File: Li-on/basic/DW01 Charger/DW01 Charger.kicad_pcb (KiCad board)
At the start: 2 copper layers, 34.5 x 20.5 mm, 10 parts, among them J1 Pos Batt, J2 NEG Batt, J3 POS IN/OUT, J4 NEG IN/OUT, Q1 RE1C002UNTCL, Q2 RE1C001ZPTL, U1 DW01A

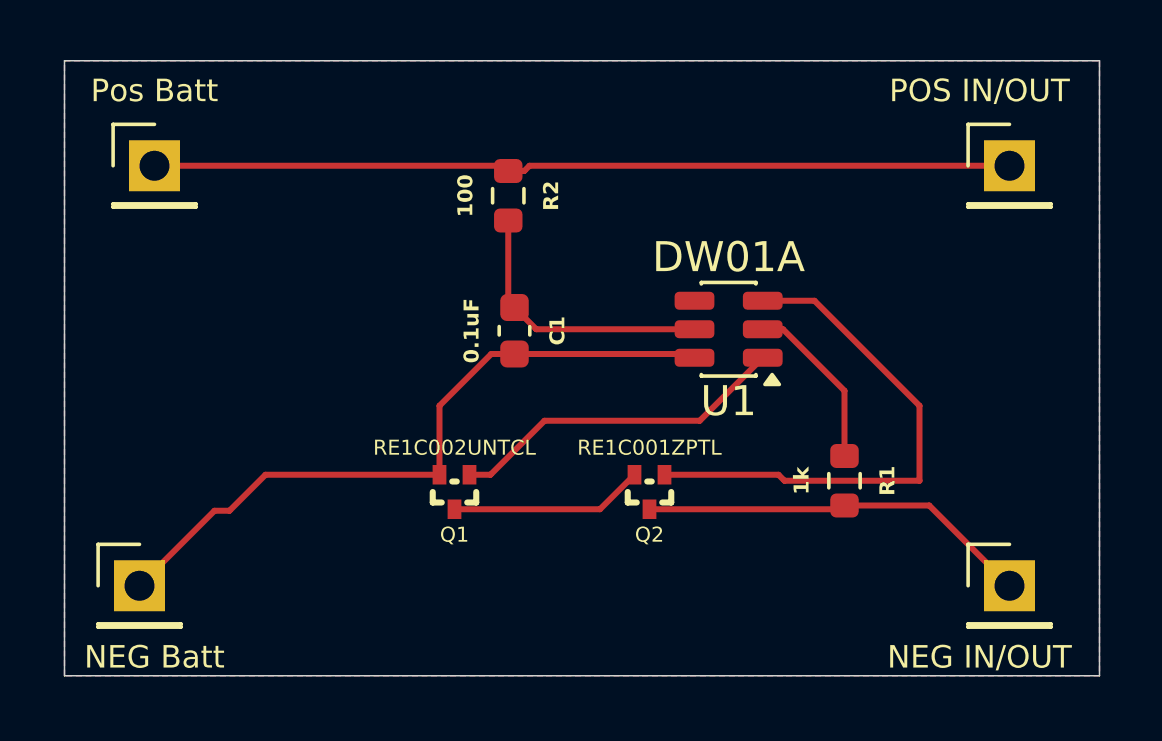
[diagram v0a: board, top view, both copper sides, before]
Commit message: hi
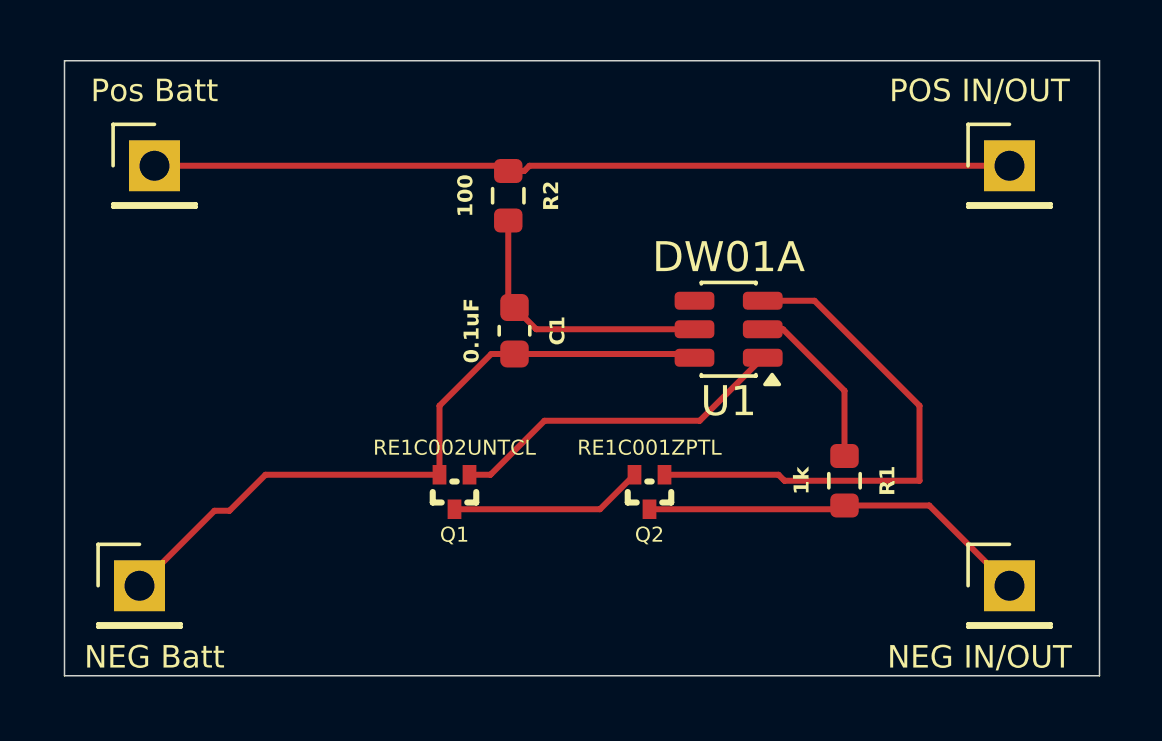
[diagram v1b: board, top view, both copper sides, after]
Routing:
- removed copper zone on B.Cu, net (none)
- removed copper zone on F.Cu, net (none)
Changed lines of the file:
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@@
 		(tenting front back)
 		(pcbplotparams
-			(layerselection 0x00000000_00000000_55555555_575555ff)
-			(plot_on_all_layers_selection 0x00000000_00000000_00000002_2200080f)
-			(disableapertmacros no)
+			(layerselection 0x00000000_00000000_55555555_57555573)
+			(plot_on_all_layers_selection 0x00000000_00000000_00000000_00000000)
+			(disableapertmacros yes)
 			(usegerberextensions yes)
 			(usegerberattributes yes)
@@
 			(layer "F.Fab")
 		)
-		(fp_text user "${REFERENCE}"
-			(at 0 0 90)
-			(layer "F.Fab")
-			(effects
-				(font
-					(size 1 1)
-					(thickness 0.15)
-				)
-			)
-		)
-		(pad "1" thru_hole rect
+		(pad "" thru_hole rect
 			(at 0 0)
 			(size 1.7 1.7)
@@
 			(layers "*.Cu" "*.Mask")
 			(remove_unused_layers no)
-			(net 3 "Net-(J1-Pad1)")
 			(pintype "passive")
 		)
@@
 			(fill no)
 			(layer "F.Fab")
-		)
-		(fp_text user "${REFERENCE}"
-			(at 0 0 0)
-			(layer "F.Fab")
-			(effects
-				(font
-					(size 0.72 0.72)
-					(thickness 0.11)
-				)
-			)
 		)
 		(pad "1" smd roundrect
@@
 			(layer "F.Fab")
 		)
-		(fp_text user "${REFERENCE}"
-			(at 0 0 90)
-			(layer "F.Fab")
-			(effects
-				(font
-					(size 1 1)
-					(thickness 0.15)
-				)
-			)
-		)
-		(pad "1" thru_hole rect
+		(pad "" thru_hole rect
 			(at 0 0)
 			(size 1.7 1.7)
@@
 			(layers "*.Cu" "*.Mask")
 			(remove_unused_layers no)
-			(net 3 "Net-(J1-Pad1)")
 			(pintype "passive")
 		)
@@
 			(layer "F.Fab")
 		)
-		(fp_text user "${REFERENCE}"
-			(at 0 0 90)
-			(layer "F.Fab")
-			(effects
-				(font
-					(size 1 1)
-					(thickness 0.15)
-				)
-			)
-		)
-		(pad "1" thru_hole rect
+		(pad "" thru_hole rect
 			(at 0 0)
 			(size 1.7 1.7)
@@
 			(layers "*.Cu" "*.Mask")
 			(remove_unused_layers no)
-			(net 1 "Net-(Q1-S)")
 			(pintype "passive")
 		)
@@
 			(layer "F.Fab")
 		)
-		(fp_text user "${REFERENCE}"
-			(at 0 0 90)
-			(layer "F.Fab")
-			(effects
-				(font
-					(size 1 1)
-					(thickness 0.15)
-				)
-			)
-		)
-		(pad "1" thru_hole rect
+		(pad "" thru_hole rect
 			(at 0 0)
 			(size 1.7 1.7)
@@
 			(layers "*.Cu" "*.Mask")
 			(remove_unused_layers no)
-			(net 4 "Net-(Q2-D)")
 			(pintype "passive")
 		)
@@
 		(net 8)
 	)
-	(zone
-		(net 0)
-		(net_name "")
-		(layer "F.Cu")
-		(name "GND")
-		(hatch edge 0.5)
-		(connect_pads yes
-			(clearance 0.5)
-		)
-		(min_thickness 0.25)
-		(filled_areas_thickness no)
-		(fill yes
-			(thermal_gap 0.5)
-			(thermal_bridge_width 0.5)
-			(island_removal_mode 1)
-			(island_area_min 10)
-		)
-		(polygon
-			(pts
-				(xy 101.5 39.5) (xy 136 39.5) (xy 136 60) (xy 101.5 60)
-			)
-		)
-	)
-	(zone
-		(net 0)
-		(net_name "")
-		(layer "B.Cu")
-		(name "GND")
-		(hatch edge 0.5)
-		(priority 1)
-		(connect_pads yes
-			(clearance 0.5)
-		)
-		(min_thickness 0.25)
-		(filled_areas_thickness no)
-		(fill yes
-			(thermal_gap 0.5)
-			(thermal_bridge_width 0.5)
-			(island_removal_mode 1)
-			(island_area_min 10)
-		)
-		(polygon
-			(pts
-				(xy 101.5 39.5) (xy 136 39.5) (xy 136 60) (xy 101.5 60)
-			)
-		)
-	)
 	(embedded_fonts no)
